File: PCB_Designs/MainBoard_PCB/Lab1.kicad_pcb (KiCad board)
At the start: 2 copper layers, 113.5 x 55.6 mm, 78 parts, among them K1 XLR3, P1 CONN_01X06, P2 USB_B, P3 CONN_02X05, P4 CONN_01X02, P5 CONN_02X05, P6 CONN_02X05, Q1 BSS138, Q2 BSS138, Q3 BSS138, Q4 BSS138, Q5 BSS138, Q6 BSS138, Q7 BSS138, U1 STM32F411RETx, U10 24C16, U2 TRACO_POWER_TEL_2-0511, U3 6N137, U4 6N137, U5 6N137, U6 FT232RL, U7 MAX481CSA, U8 UA78M05IDCY, U9 UA78M33CDCY, Y1 8MHz

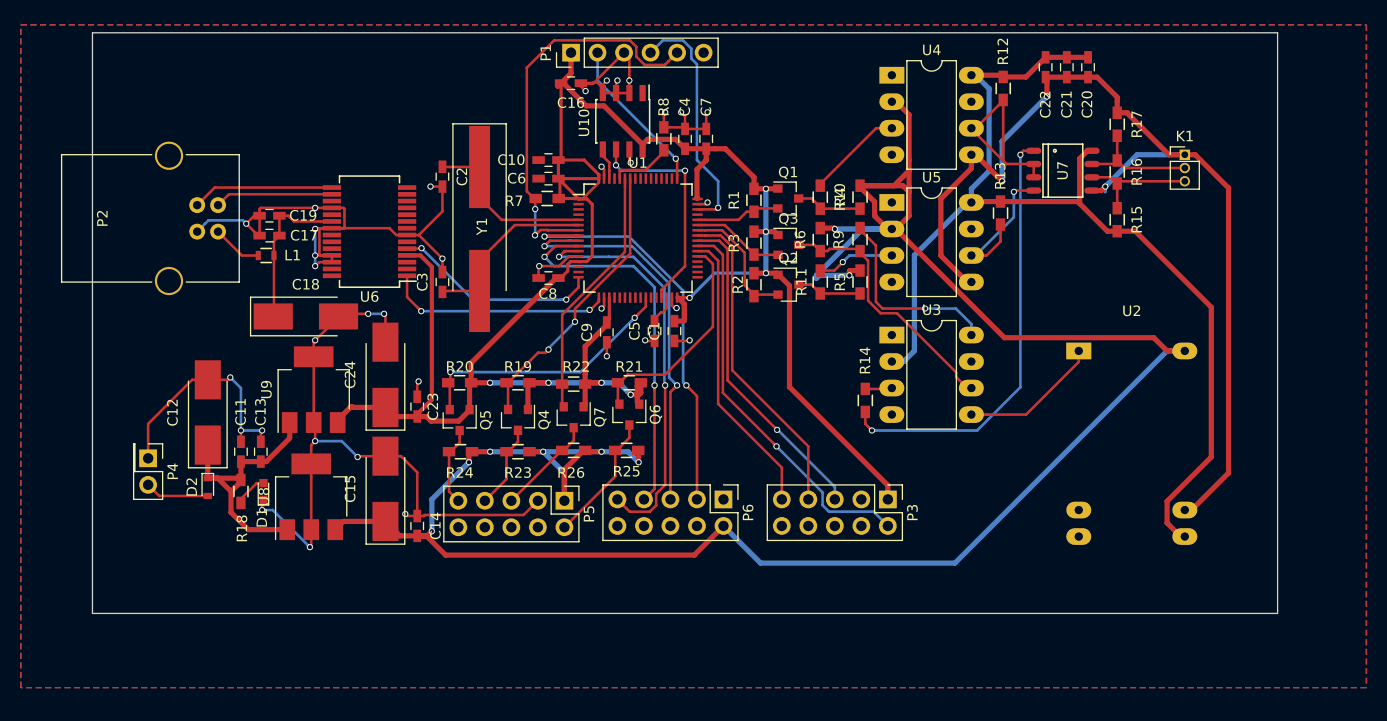
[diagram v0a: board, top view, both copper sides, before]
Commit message: Main_PCB V1 Complete
Minor changes to everything.
Main_PCB complete with traces and design.
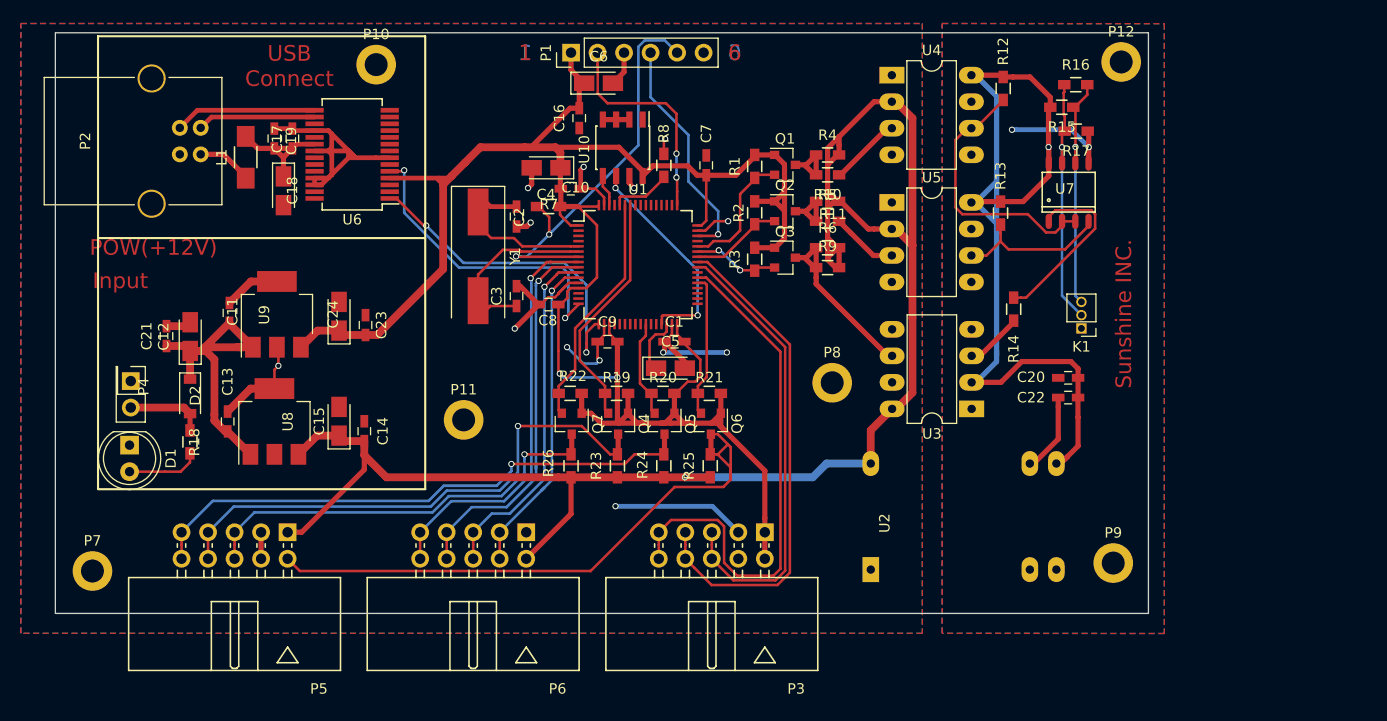
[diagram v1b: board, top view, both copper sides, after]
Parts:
- added P10: CONN_01X01, Mounting_Holes:MountingHole_2.2mm_M2_DIN965_Pad, F.Cu at (65.8, 47.8)
- added P11: CONN_01X01, Mounting_Holes:MountingHole_2.2mm_M2_DIN965_Pad, F.Cu at (74.2, 81.8)
- added P12: CONN_01X01, Mounting_Holes:MountingHole_2.2mm_M2_DIN965_Pad, F.Cu at (137.2, 47.5)
- added P7: CONN_01X01, Mounting_Holes:MountingHole_2.2mm_M2_DIN965_Pad, F.Cu at (38.6, 96.3)
- added P8: CONN_01X01, Mounting_Holes:MountingHole_2.2mm_M2_DIN965_Pad, F.Cu at (109.5, 78.2)
- added P9: CONN_01X01, Mounting_Holes:MountingHole_2.2mm_M2_DIN965_Pad, F.Cu at (136.4, 95.5)
- C12, C15, C18, C24: footprint Capacitors_Tantalum_SMD:CP_Tantalum_Case-C_EIA-6032-28_Hand -> Capacitors_Tantalum_SMD:CP_Tantalum_Case-A_EIA-3216-18_Reflow
- C4: value 100n -> 4.7u; footprint Capacitors_SMD:C_0603_HandSoldering -> Capacitors_Tantalum_SMD:CP_Tantalum_Case-A_EIA-3216-18_Reflow
- C5, C6: footprint Capacitors_SMD:C_0603_HandSoldering -> Capacitors_Tantalum_SMD:CP_Tantalum_Case-A_EIA-3216-18_Reflow
- D1: footprint LEDs:LED_0603 -> LEDs:LED_D5.0mm
- D2: footprint Diodes_SMD:D_0603 -> Diodes_SMD:D_SOD-123
- L1: footprint Resistors_SMD:R_0603 -> Resistors_SMD:R_1206_HandSoldering
- P3, P5, P6: footprint Pin_Headers:Pin_Header_Straight_2x05_Pitch2.54mm -> Connectors_Multicomp:Multicomp_MC9A22-1034_2x05x2.54mm_Angled
- Y1: footprint Crystals:Crystal_SMD_HC49-SD_HandSoldering -> Crystals:Crystal_SMD_HC49-SD
- moved C21 90.0 mm to (45.7, 73.8), turned to 90 degrees
- moved C22 31.7 mm to (132.1, 79.7), turned to 180 degrees
- moved C20 29.8 mm to (132.1, 77.8), turned to 180 degrees
- moved U2 28.9 mm to (113.2, 96.1), turned to 90 degrees
- moved P5 26.7 mm to (57.3, 92.6), turned to 180 degrees
- moved Q5 19.6 mm to (93.4, 82.2)
- moved R24 19.5 mm to (93.3, 86.2), turned to 270 degrees
- moved R20 19.5 mm to (93.3, 79.2)
- moved K1 19.4 mm to (133.3, 73.0), turned to 180 degrees
- moved P6 19.2 mm to (80.2, 92.6), turned to 180 degrees
- moved R14 16.7 mm to (126.9, 71.2), turned to 270 degrees
- moved C4 13.6 mm to (82.1, 57.6), turned to 180 degrees
- moved D1 13.6 mm to (42.2, 84.2), turned to 270 degrees
- moved C11 13.3 mm to (51.7, 71.5)
- moved C18 12.2 mm to (56.9, 59.8), turned to 270 degrees
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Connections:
- C11 pad 1: +12V -> Net-(C11-Pad1)
- C12 pad 1: +12V -> Net-(C11-Pad1)
- C13 pad 1: +12V -> Net-(C11-Pad1)
- C21 pad 1: /VDD5EXT -> Net-(C11-Pad1)
- C21 pad 2: /GNDEXT -> GND
- C4 pad 1: GND -> +3V3
- C4 pad 2: +3V3 -> GND
- C5 pad 1: GND -> Net-(C5-Pad1)
- C5 pad 2: Net-(C5-Pad2) -> GND
- C6 pad 1: GND -> +3V3
- C6 pad 2: +3V3 -> GND
- D2 pad 1: +12V -> Net-(C11-Pad1)
- D2 pad 2: Net-(D2-Pad2) -> +12V
- P1 pad 6: Net-(P1-Pad6) -> (no net)
- P3 pad 10: Net-(P3-Pad10) -> /INT_BUTTA
- P3 pad 2: /INT_BUTTB -> +3V3
- P3 pad 4: Net-(P3-Pad4) -> GND
- P3 pad 6: Net-(P3-Pad6) -> /BUTT_I2C_SDA
- P3 pad 8: Net-(P3-Pad8) -> /BUTT_I2C_SCL
- P4 pad 2: Net-(D2-Pad2) -> +12V
- P5 pad 4: Net-(P5-Pad4) -> GND
- P5 pad 6: Net-(P5-Pad6) -> Net-(P5-Pad5)
- P5 pad 8: Net-(P5-Pad8) -> Net-(P5-Pad7)
- P5 pad 9: Net-(P5-Pad9) -> Net-(P5-Pad10)
- P6 pad 4: Net-(P6-Pad4) -> Net-(P6-Pad3)
- P6 pad 6: Net-(P6-Pad6) -> Net-(P6-Pad5)
- P6 pad 8: Net-(P6-Pad8) -> Net-(P6-Pad7)
- P6 pad 9: Net-(P6-Pad9) -> Net-(P6-Pad10)
- Q5 pad 3: Net-(P5-Pad9) -> Net-(P5-Pad10)
- R24 pad 1: Net-(P5-Pad9) -> Net-(P5-Pad10)
- R9 pad 1: Net-(R9-Pad1) -> +5V
- U1 pad 10: Net-(P6-Pad7) -> Net-(P6-Pad5)
- U1 pad 11: Net-(P6-Pad9) -> Net-(P6-Pad3)
- U1 pad 14: Net-(U1-Pad14) -> (no net)
- U1 pad 15: Net-(U1-Pad15) -> (no net)
- U1 pad 2: Net-(U1-Pad2) -> (no net)
- U1 pad 20: Net-(U1-Pad20) -> (no net)
- U1 pad 21: Net-(U1-Pad21) -> (no net)
- U1 pad 22: Net-(U1-Pad22) -> (no net)
- U1 pad 23: Net-(U1-Pad23) -> (no net)
- U1 pad 24: Net-(U1-Pad24) -> (no net)
- U1 pad 25: Net-(U1-Pad25) -> (no net)
- U1 pad 27: Net-(U1-Pad27) -> (no net)
- U1 pad 28: Net-(U1-Pad28) -> (no net)
- U1 pad 3: Net-(U1-Pad3) -> (no net)
- U1 pad 30: Net-(C5-Pad2) -> Net-(C5-Pad1)
- U1 pad 33: Net-(U1-Pad33) -> (no net)
- U1 pad 34: Net-(U1-Pad34) -> (no net)
- U1 pad 35: Net-(U1-Pad35) -> (no net)
- U1 pad 36: Net-(U1-Pad36) -> (no net)
- U1 pad 39: /INT_BUTTB -> (no net)
- U1 pad 4: Net-(U1-Pad4) -> (no net)
- U1 pad 45: Net-(U1-Pad45) -> (no net)
- U1 pad 50: Net-(U1-Pad50) -> (no net)
- U1 pad 51: Net-(U1-Pad51) -> (no net)
- U1 pad 52: Net-(U1-Pad52) -> (no net)
- U1 pad 53: Net-(U1-Pad53) -> (no net)
- U1 pad 54: Net-(U1-Pad54) -> (no net)
- U1 pad 55: Net-(U1-Pad55) -> (no net)
- U1 pad 56: Net-(U1-Pad56) -> (no net)
- U1 pad 57: Net-(U1-Pad57) -> (no net)
- U1 pad 61: Net-(U1-Pad61) -> (no net)
- U1 pad 8: Net-(P6-Pad3) -> Net-(P6-Pad10)
- U1 pad 9: Net-(P6-Pad5) -> Net-(P6-Pad7)
- U10 pad 1: Net-(U10-Pad1) -> (no net)
- U2 pad 7: Net-(U2-Pad7) -> (no net)
- U2 pad 8: Net-(U2-Pad8) -> (no net)
- U3 pad 7: Net-(U3-Pad7) -> (no net)
- U3 pad 8: Net-(R9-Pad1) -> +5V
- U4 pad 7: Net-(U4-Pad7) -> (no net)
- U5 pad 7: Net-(U5-Pad7) -> (no net)
- U6 pad 10: Net-(U6-Pad10) -> (no net)
- U6 pad 11: Net-(U6-Pad11) -> (no net)
- U6 pad 12: Net-(U6-Pad12) -> (no net)
- U6 pad 13: Net-(U6-Pad13) -> (no net)
- U6 pad 14: Net-(U6-Pad14) -> (no net)
- U6 pad 17: Net-(U6-Pad17) -> (no net)
- U6 pad 19: Net-(U6-Pad19) -> (no net)
- U6 pad 2: Net-(U6-Pad2) -> (no net)
- U6 pad 22: Net-(U6-Pad22) -> (no net)
- U6 pad 23: Net-(U6-Pad23) -> (no net)
- U6 pad 27: Net-(U6-Pad27) -> (no net)
- U6 pad 28: Net-(U6-Pad28) -> (no net)
- U6 pad 3: Net-(U6-Pad3) -> (no net)
- U6 pad 6: Net-(U6-Pad6) -> (no net)
- U6 pad 9: Net-(U6-Pad9) -> (no net)
- U8 pad 1: +12V -> Net-(C11-Pad1)
- U9 pad 1: +12V -> Net-(C11-Pad1)
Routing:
- net GND: track 203.7 -> 116.7 mm, vias 35 -> 13
- net /GNDEXT: track 97.8 -> 20.8 mm, vias 3 -> 2
- net +5V: track 221.2 -> 161.0 mm, vias 8 -> 1
- net Net-(P5-Pad10): track 0.00 -> 54.2 mm, vias 0 -> 1
- net Net-(P5-Pad2): track 12.6 -> 59.1 mm
- net Net-(P5-Pad7): track 8.57 -> 51.8 mm, vias 0 -> 1
- net Net-(P6-Pad9): track 39.8 -> 0.00 mm, vias 2 -> 0
- net Net-(P6-Pad10): track 0.00 -> 39.7 mm, vias 0 -> 1
- net /INT_BUTTB: track 37.8 -> 0.00 mm, vias 1 -> 0
- net Net-(C11-Pad1): track 0.00 -> 33.2 mm
- net Net-(P5-Pad5): track 9.74 -> 40.9 mm, vias 0 -> 1
- net Net-(R14-Pad1): track 41.7 -> 17.6 mm, vias 2 -> 0
- net /INT_BUTTA: track 27.7 -> 50.9 mm
- net +12V: track 27.6 -> 7.54 mm
- net Net-(R9-Pad1): track 18.8 -> 0.00 mm, vias 1 -> 0
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- added copper zone on B.Cu, net /GNDEXT
- added copper zone on F.Cu, net /GNDEXT
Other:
- board size 113.5 x 55.6 mm -> 104.7 x 55.6 mm
- net class Default: clearance 0.2 -> 0.15
- net class Power: clearance 0.2 -> 0.15
- rule trace_clearance: 0.2 -> 0.15
- board text added: "1"
- board text added: "6"
- board text added: "Input"
- board text added: "POW(+12V)"
- board text added: "Sunshine INC."
- board text added: "USB Connect"
